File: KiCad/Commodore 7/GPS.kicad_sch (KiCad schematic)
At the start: 4 parts, among them IC1 BGU7004,115, U2 NEO-M9N-00B

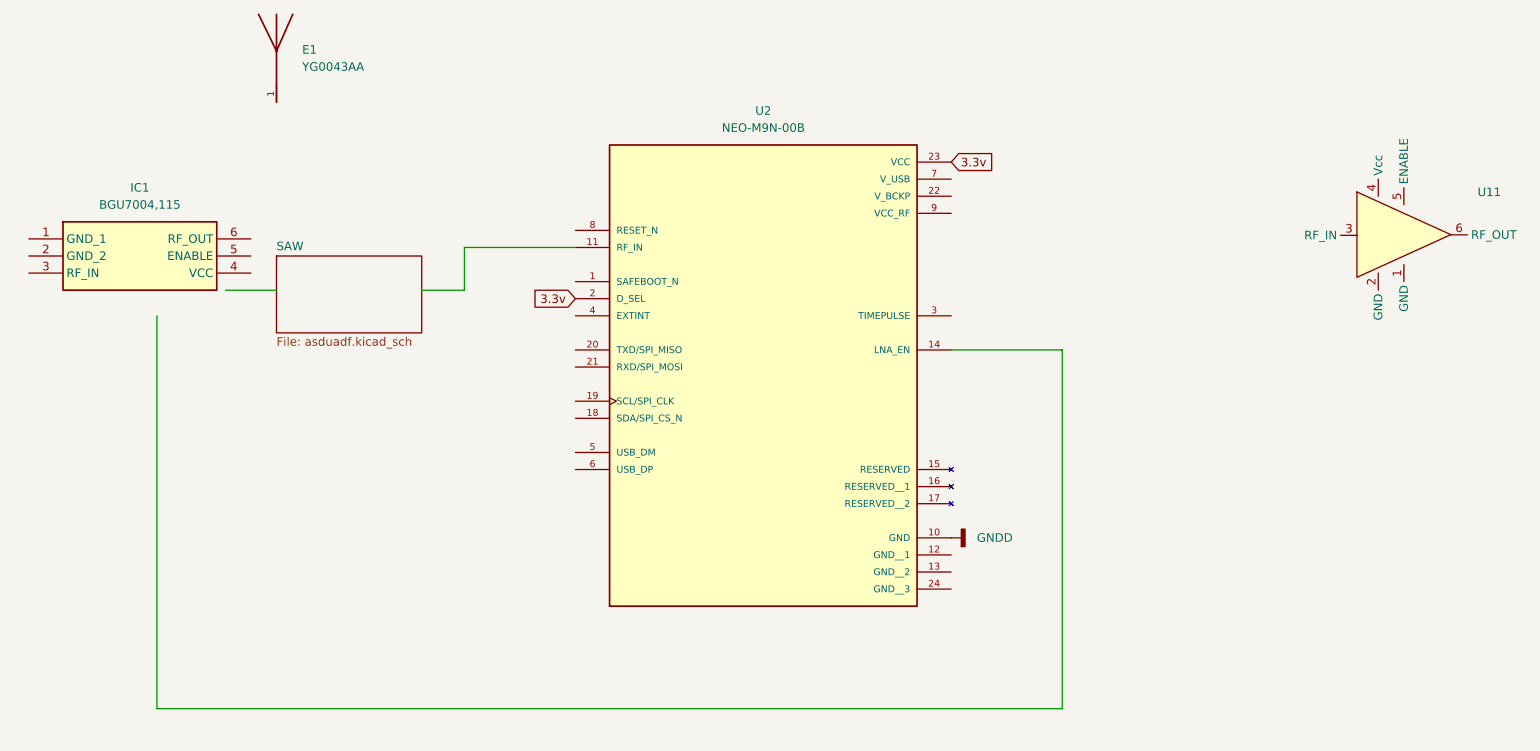
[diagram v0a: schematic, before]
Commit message: started pcb design
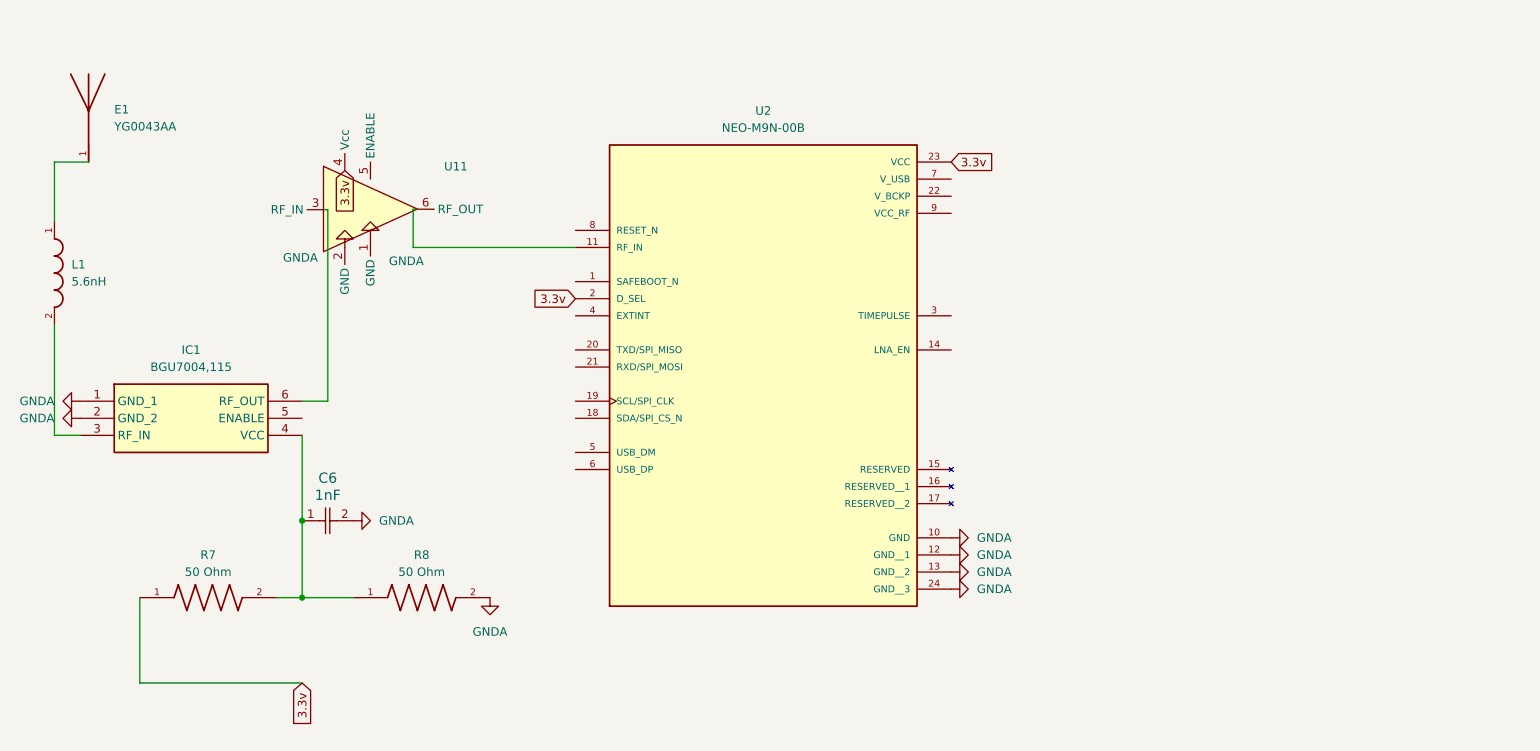
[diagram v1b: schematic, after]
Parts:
- added C6: 1nF, CC0603KRXQRQBB104:CC0603N_YAG, symbol CC0603KRX7R7BB104:CC0603KRX7R7BB104
- added L1: 5.6nH, LQW15AN5N6G80D:INDC1006X60N, symbol LQW15AN5N6G80D:LQW15AN5N6G80D
- added R7, R8: 50 Ohm, RT0402BRE0750RL:RESC1005X35N, symbol RT0402BRE0750RL:RT0402BRE0750RL
- U11: footprint SOT-886 -> Package_TO_SOT_SMD:SOT-886
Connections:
- net GNDD is gone; now on net GNDA: U2.10 (GND)
- net 3.3v: now also U11.4 (Vcc), R7.1
- net GNDA: now reaches IC1.1 (GND_1)
- net GNDA: now also IC1.2 (GND_2), U11.1 (GND), U11.2 (GND), U2.12 (GND__1), U2.13 (GND__2), U2.24 (GND__3), C6.2, R8.2
- net at IC1.3 (RF_IN): now also L1.2
- net at IC1.4 (VCC): now also C6.1, R7.2, R8.1
- net at IC1.6 (RF_OUT): now also U11.3 (RF_IN)
- net at U11.6 (RF_OUT): now also U2.11 (RF_IN)
- net at E1.1: now also L1.1
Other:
- removed sheet SAW
- moved on the sheet: E1, IC1, U11

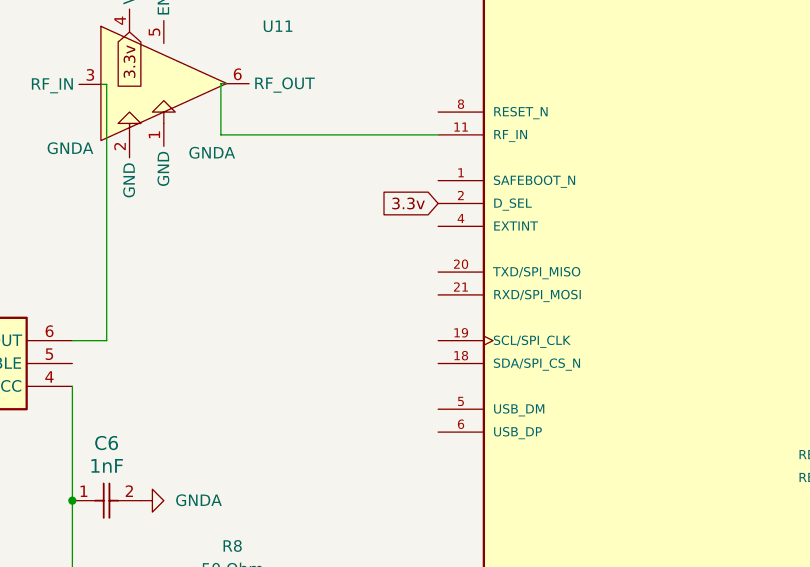
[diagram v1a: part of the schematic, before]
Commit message: uhhhhhhhh idk
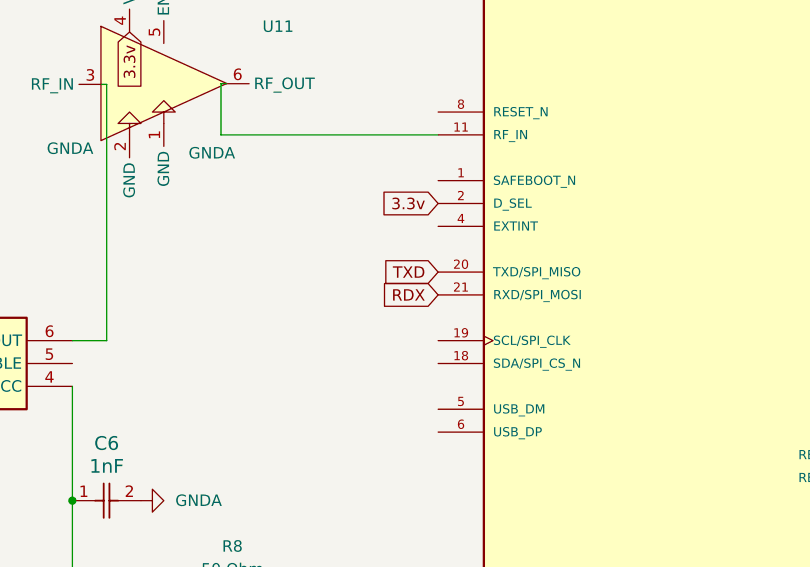
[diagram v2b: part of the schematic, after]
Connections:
- net TXD: now reaches U2.20 (TXD/SPI_MISO)
- net RDX: now reaches U2.21 (RXD/SPI_MOSI)
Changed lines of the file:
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@@
+		)
+	)
+	(global_label "TXD"
+		(shape input)
+		(at 95.25 92.71 180)
+		(fields_autoplaced yes)
+		(effects
+			(font
+				(size 1.27 1.27)
+			)
+			(justify right)
+		)
+		(property "Intersheetrefs" "${INTERSHEET_REFS}"
+			(at 88.8177 92.71 0)
+			(effects
+				(font
+					(size 1.27 1.27)
+				)
+				(justify right)
+				(hide yes)
+			)
 		)
 	)
@@
 				(hide yes)
 			)
+		)
+	)
+	(global_label "RDX"
+		(shape input)
+		(at 95.25 95.25 180)
+		(fields_autoplaced yes)
+		(effects
+			(font
+				(size 1.27 1.27)
+			)
+			(justify right)
+		)
+		(property "Intersheetrefs" "${INTERSHEET_REFS}"
+			(at 88.5153 95.25 0)
+			(effects
+				(font
+					(size 1.27 1.27)
+				)
+				(justify right)
+				(hide yes)
+			)

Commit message: i sitll got mroe to do ssry yall
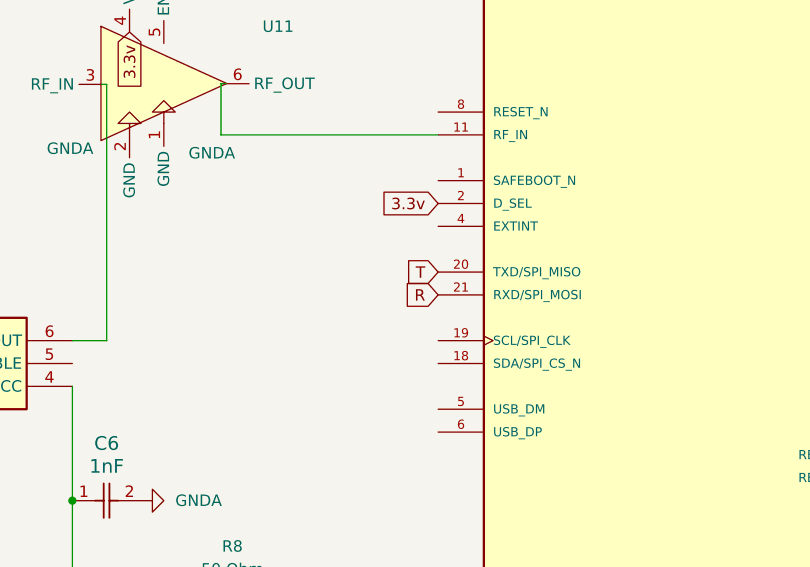
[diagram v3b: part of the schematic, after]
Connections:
- net RDX renamed R
- net TXD renamed T
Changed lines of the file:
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@@
 		)
 	)
-	(global_label "TXD"
+	(global_label "T"
 		(shape input)
 		(at 95.25 92.71 180)
@@
 		)
 		(property "Intersheetrefs" "${INTERSHEET_REFS}"
-			(at 88.8177 92.71 0)
+			(at 91.2972 92.71 0)
 			(effects
 				(font
@@
 		)
 	)
-	(global_label "RDX"
+	(global_label "R"
 		(shape input)
 		(at 95.25 95.25 180)
@@
 		)
 		(property "Intersheetrefs" "${INTERSHEET_REFS}"
-			(at 88.5153 95.25 0)
+			(at 90.9948 95.25 0)
 			(effects
 				(font
